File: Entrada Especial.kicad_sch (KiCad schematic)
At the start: 0 parts

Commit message: 15-may-26
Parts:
- added C141, C142, C143, C146, C148, C151, C152, C153, C154, C155, C156: 0.1uF, Capacitor_SMD:C_0603_1608Metric_Pad1.08x0.95mm_HandSolder, symbol Device:C_Small
- added C144: 22uF, symbol Device:C_Small
- added C145: 470nF, Capacitor_SMD:C_0603_1608Metric, symbol Device:C_Small
- added C147, C150: 4.7uF, Capacitor_SMD:C_0603_1608Metric, symbol Device:C_Small
- added C149: 10uF, Capacitor_SMD:C_0603_1608Metric, symbol Device:C_Small
- added D36: LED, LED_SMD:LED_0402_1005Metric, symbol Device:LED
- added D37, D40: BZV55B11, Diode_SMD:D_MiniMELF, symbol Diode:BZV55B11
- added D38, D39: BZV55B3V3, Diode_SMD:D_MiniMELF, symbol Diode:BZV55B3V3
- added IC16, IC17: ILD206T, SOIC:SOIC 8, symbol OPTOACOPLADORES:ILD206T
- added J*3: 1728840000, CONECTORES GRACIDA:16POS-2LINEAS-3.5PITCH, symbol CONECTORES GRACIDA:Weidmüller 1728840000 16pos P3.5mm socket
- added L17: L_Iron_Small, symbol Device:L_Iron_Small
- added L20: 0603, Inductor_SMD:L_0603_1608Metric_Pad1.05x0.95mm_HandSolder, symbol Device:L_Iron_Small
- added R239, R246: 10k, Resistor_SMD:R_0603_1608Metric, symbol Device:R_US
- added R240, R241, R242, R243, R247, R248, R249, R250, R251, R252, R253, R254, R255, R256, R257, R258, R259, R260, R261, R262, R263, R264, R265, R266: 10, Resistor_SMD:R_0603_1608Metric, symbol Device:R_US
- added R244: 100, Resistor_SMD:R_0603_1608Metric_Pad0.98x0.95mm_HandSolder, symbol Device:R_Small_US
- added R245: 1k, Resistor_SMD:R_0603_1608Metric_Pad0.98x0.95mm_HandSolder, symbol Device:R_Small_US
- added R267, R268, R269, R270: 2.2k, Capacitor_SMD:C_0603_1608Metric_Pad1.08x0.95mm_HandSolder, symbol Device:R_Small_US
- added R271, R272, R273, R275: 4.7k, Capacitor_SMD:C_0603_1608Metric_Pad1.08x0.95mm_HandSolder, symbol Device:R_Small_US
- added TH3: B59985C120A70, TERMISTORES GRACIDA:B59985C0120A070, symbol Device:Thermistor_PTC
- added U32, U35: TLV9301xDBV, Package_TO_SOT_SMD:SOT-23-5, symbol Amplifier_Operational:TLV9301xDBV
- added U33: LM7705, Package_SO:VSSOP-8_3x3mm_P0.65mm, symbol Regulator_SwitchedCapacitor:LM7705
- added U34: MCP1799T-5002H/TT, Package_TO_SOT_SMD:SOT-23, symbol Regulator_Linear:MCP1799x-500xxTT
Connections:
- new net: IC17.1 (A_1), R269.2
- new net: IC17.3 (A_2), R270.2
- new net: R248.1, R250.2
- new net: R248.2, R249.1
- new net: R254.1, R256.2
- new net: R253.1, R254.2, R255.1, R257.1
- new net: R263.2, R264.1
- new net: R262.1, R264.2, R265.1, R266.1
- new net: C141.2, L17.2, TH3.1
- new net: R240.1, R241.1, U35.1
- new net: R250.1, R252.1, R253.2
- new net: C150.1, C151.2, U33.1 (CF+)
- new net: C150.2, C151.1, U33.8 (CF-)
- new net: R241.2, R242.2
- new net: C144.1, C145.1, L20.1, U33.6 (VOUT)
- new net: C143.1, L20.2, U32.2 (V-), U35.2 (V-)
- new net: J*3. (9), R269.1
- new net: R247.1, R251.1, U32.1
- new net: R258.2, U32.3 (+)
- new net: R252.2, U32.4 (-)
- new net: C148.2, C149.1, C152.2, D36.2 (A), U33.4 (VDD), U34.2 (VO)
- new net: R260.2, U35.3 (+)
- new net: R259.2, U35.4 (-)
- new net: C146.2, C147.1, U33.7 (CRES)
- new net: R259.1, R261.1, R262.2
- new net: R243.1, R261.2
- new net: R249.2, R251.2
- new net: D40.1 (K), J*3. (9), R260.1
- new net: IC16.1 (A_1), R267.2
- new net: IC16.3 (A_2), R268.2
- new net: D36.1 (K), R245.1
- new net: J*3. (9), R270.1
- new net: D37.1 (K), J*3. (9), R258.1
- new net: R244.1, U33.3 (SD)
- new net: J*3. (9), R268.1
- new net: R242.1, R243.2
- new net +12V: C153.2, C154.1, C155.1, R256.1, R263.1, U32.5 (V+), U34.3 (VI), U35.5 (V+)
- new net +24V: TH3.2
- new net +3.3V: R271.1, R272.1, R273.1, R275.1
- new net AN0_POT: D38.1 (K), R246.2, R247.2
- new net AN1_POT: D39.1 (K), R239.2, R240.2
- new net Error_Conn_Entrada_ESP+24v: C142.2, J*3. (9), L17.1, R267.1
- new net GND: C141.1, C142.1, C143.2, C144.2, C145.2, C146.1, C147.2, C148.1, C149.2, C152.1, C153.1, C154.2, C155.2, C156.2, D37.2 (A), D38.2 (A), D39.2 (A), D40.2 (A), IC16.2 (C_1), IC16.4 (C_2), IC16.5 (E_1), IC16.7 (E_2), IC17.2 (C_1), IC17.4 (C_2), IC17.5 (E_1), IC17.7 (E_2), J*3. (9), R239.1, R244.2, R245.2, R246.1, R255.2, R257.2, R265.2, R266.2, U33.2 (GND), U33.5 (GND), U34.1 (GND)
- new net opto_out1: IC16.8 (C_4), R271.2
- new net opto_out2: IC16.6 (C_3), R273.2
- new net opto_out3: IC17.8 (C_4), R272.2
- new net opto_out4: IC17.6 (C_3), R275.2
- no-connect marks 0 -> 1
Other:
- note added: "+5v"
- note added: "-0.23v"
- note added: "micro"

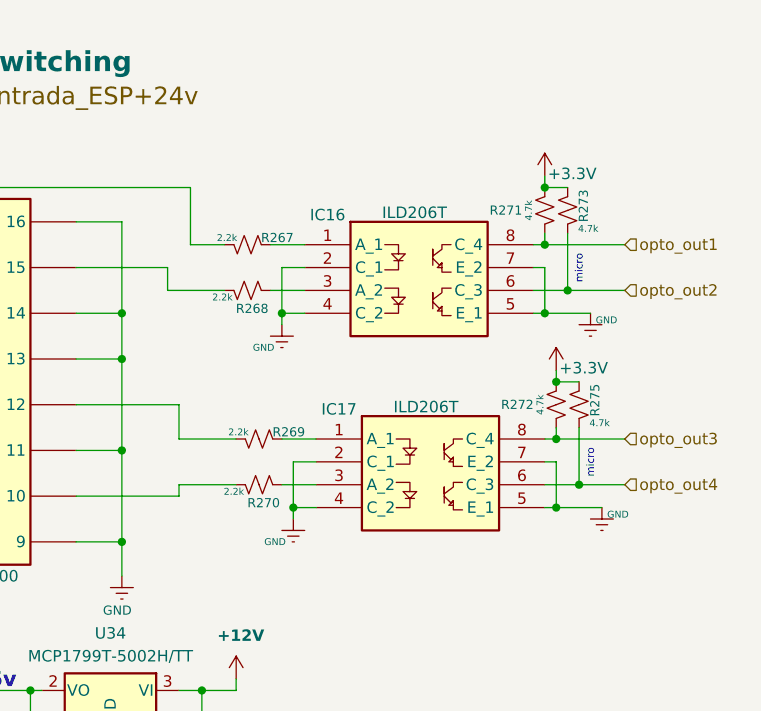
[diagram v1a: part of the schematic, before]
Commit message: pcb 18 may 26
 falta poner la fuente de +12/ ya esta casi todo
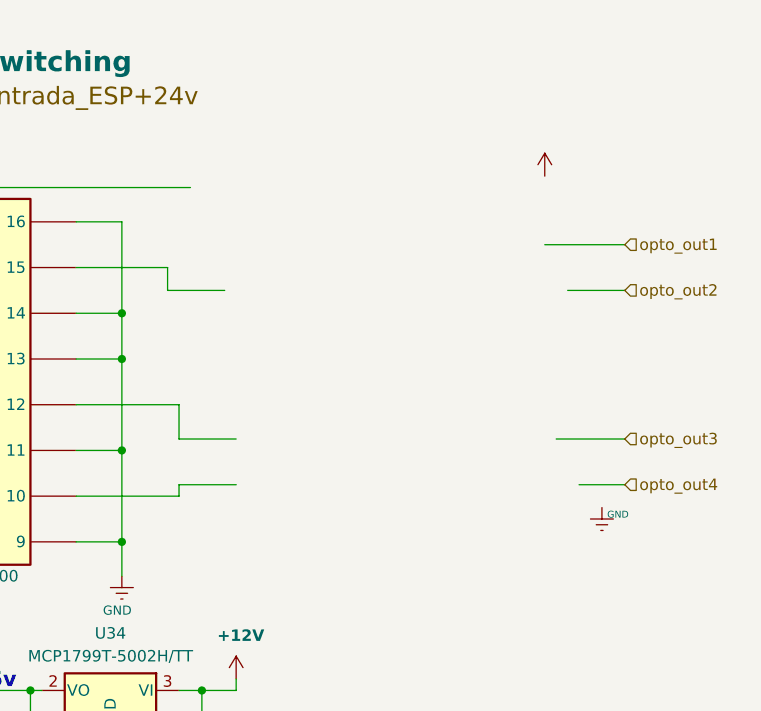
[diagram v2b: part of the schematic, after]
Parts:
- removed IC16, IC17: ILD206T, SOIC:SOIC 8, symbol OPTOACOPLADORES:ILD206T
- removed R267, R268, R269, R270: 2.2k, Capacitor_SMD:C_0603_1608Metric_Pad1.08x0.95mm_HandSolder, symbol Device:R_Small_US
- removed R271, R272, R273, R275: 4.7k, Capacitor_SMD:C_0603_1608Metric_Pad1.08x0.95mm_HandSolder, symbol Device:R_Small_US
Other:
- note removed: "micro"
